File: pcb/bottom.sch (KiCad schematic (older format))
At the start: 41 parts, among them J1 MALE, J10 TC2030_NL, J11 STANDOFF, J12 STANDOFF, J13 STANDOFF, J14 STANDOFF, J2 FEMALE, J3 MALE, J4 FEMALE, J5 MALE, J6 FEMALE, J7 MALE, J8 FEMALE, J9 DTR, Q1 PN2222A, U3 ATmega328P-MU, Y1 YSX321SL

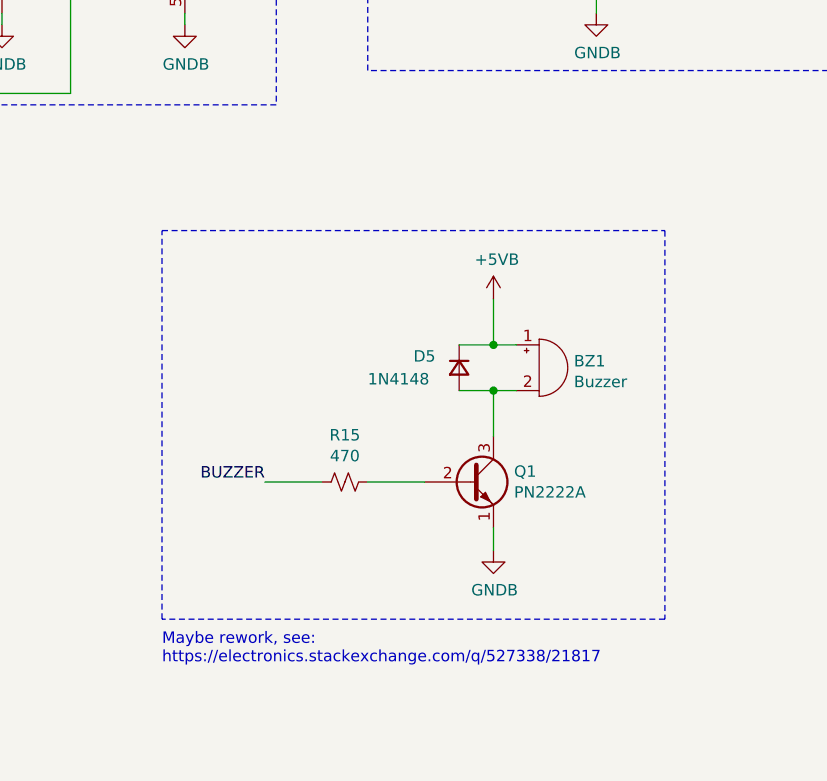
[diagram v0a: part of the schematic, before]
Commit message: Iterate
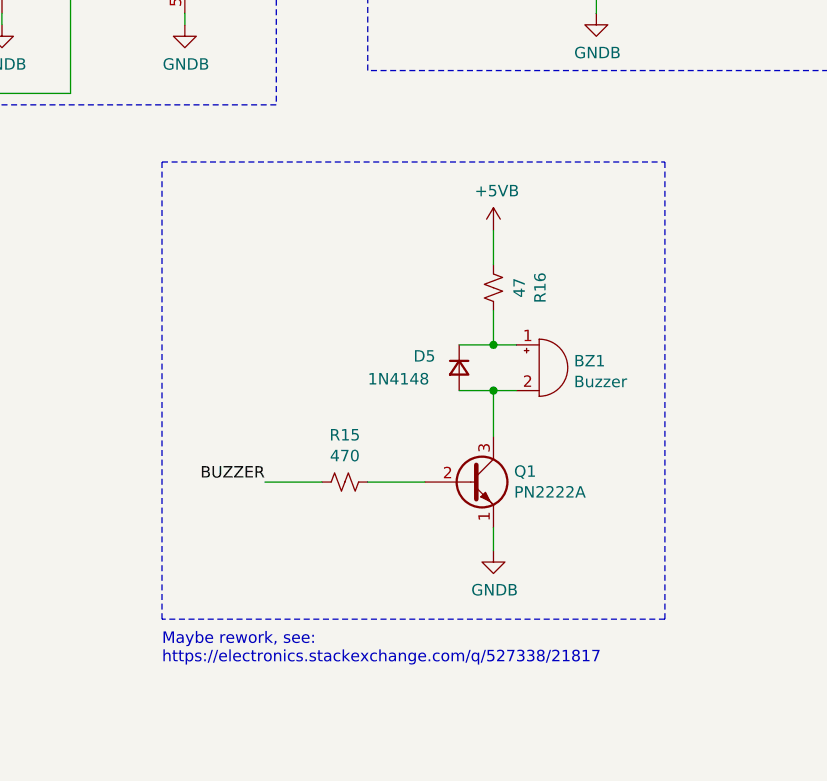
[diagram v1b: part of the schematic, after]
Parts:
- added R16: 47, Resistor_SMD:R_0402_1005Metric, symbol Device:R_Small_US
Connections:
- net +5VB: now also R16.2; no longer BZ1.1 (-), D5.1 (K)
- new net: BZ1.1 (-), D5.1 (K), R16.1
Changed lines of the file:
@@
 $Descr A4 11693 8268
 encoding utf-8
-Sheet 3 3
+Sheet 2 3
 Title "Bottom"
 Date ""
@@
 L node:+5VB #PWR01
 U 1 1 5F965E09
-P 8500 4700
-F 0 "#PWR01" H 8500 4550 50  0001 C CNN
-F 1 "+5VB" H 8515 4873 50  0000 C CNN
-F 2 "" H 8500 4700 50  0001 C CNN
-F 3 "" H 8500 4700 50  0001 C CNN
-	1    8500 4700
+P 8500 4400
+F 0 "#PWR01" H 8500 4250 50  0001 C CNN
+F 1 "+5VB" H 8515 4573 50  0000 C CNN
+F 2 "" H 8500 4400 50  0001 C CNN
+F 3 "" H 8500 4400 50  0001 C CNN
+	1    8500 4400
 	1    0    0    -1
 $EndComp
@@
 	8350 4900 8500 4900
 Wire Wire Line
-	8500 4700 8500 4900
+	8500 4750 8500 4900
 Connection ~ 8500 4900
 Wire Wire Line
 	8500 4900 8600 4900
 Wire Notes Line
-	7050 4400 9250 4400
-Wire Notes Line
-	9250 4400 9250 6100
+	7050 4100 9250 4100
+Wire Notes Line
+	9250 4100 9250 6100
 Wire Notes Line
 	9250 6100 7050 6100
 Wire Notes Line
-	7050 6100 7050 4400
+	7050 6100 7050 4100
 Text Notes 7050 6300 0    50   ~ 0
 Maybe rework, see:\nhttps://electronics.stackexchange.com/q/527338/21817
@@
 Wire Wire Line
 	2650 4900 3450 4900
+$Comp
+L Device:R_Small_US R16
+U 1 1 5F8D7356
+P 8500 4650
+F 0 "R16" V 8295 4650 50  0000 C CNN
+F 1 "47" V 8386 4650 50  0000 C CNN
+F 2 "Resistor_SMD:R_0402_1005Metric" H 8500 4650 50  0001 C CNN
+F 3 "~" H 8500 4650 50  0001 C CNN
+	1    8500 4650
+	-1   0    0    1
+$EndComp
+Wire Wire Line
+	8500 4550 8500 4400
 $EndSCHEMATC
